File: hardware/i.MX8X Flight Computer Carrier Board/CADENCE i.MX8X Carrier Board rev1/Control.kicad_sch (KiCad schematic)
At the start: 9 parts, among them SW1 SW_DIP_x04, SW2 KMR221GLFS, SW3 SW_DIP_x01

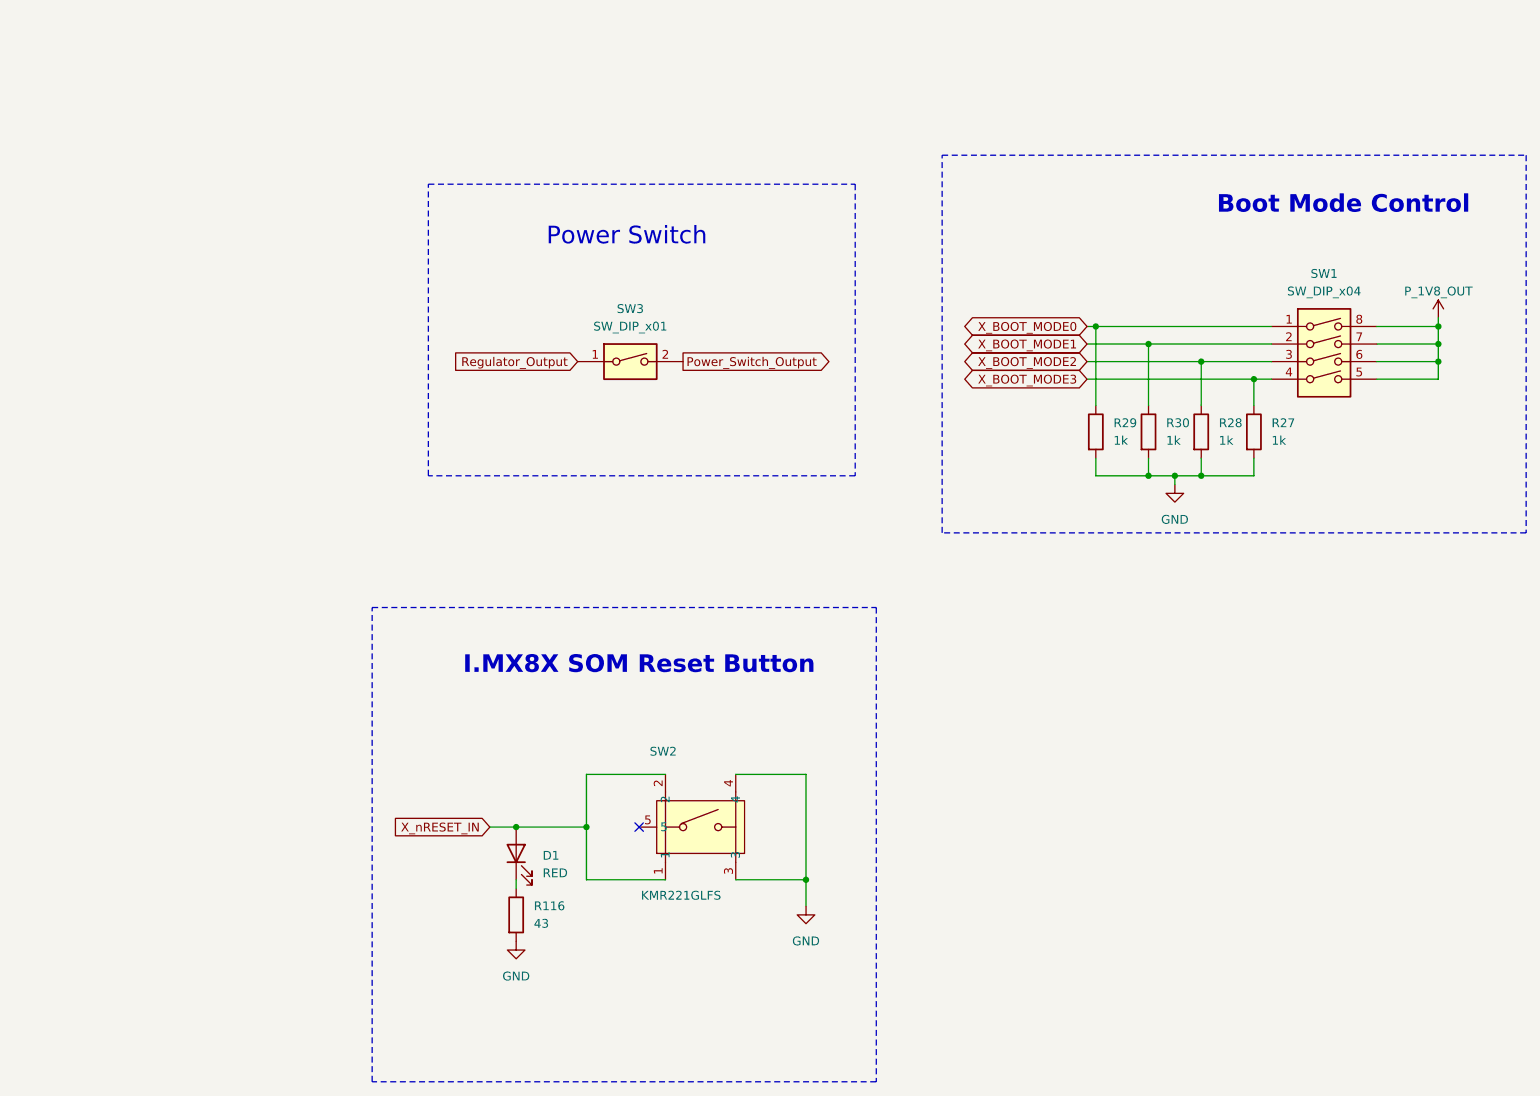
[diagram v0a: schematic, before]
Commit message: schematic reorg
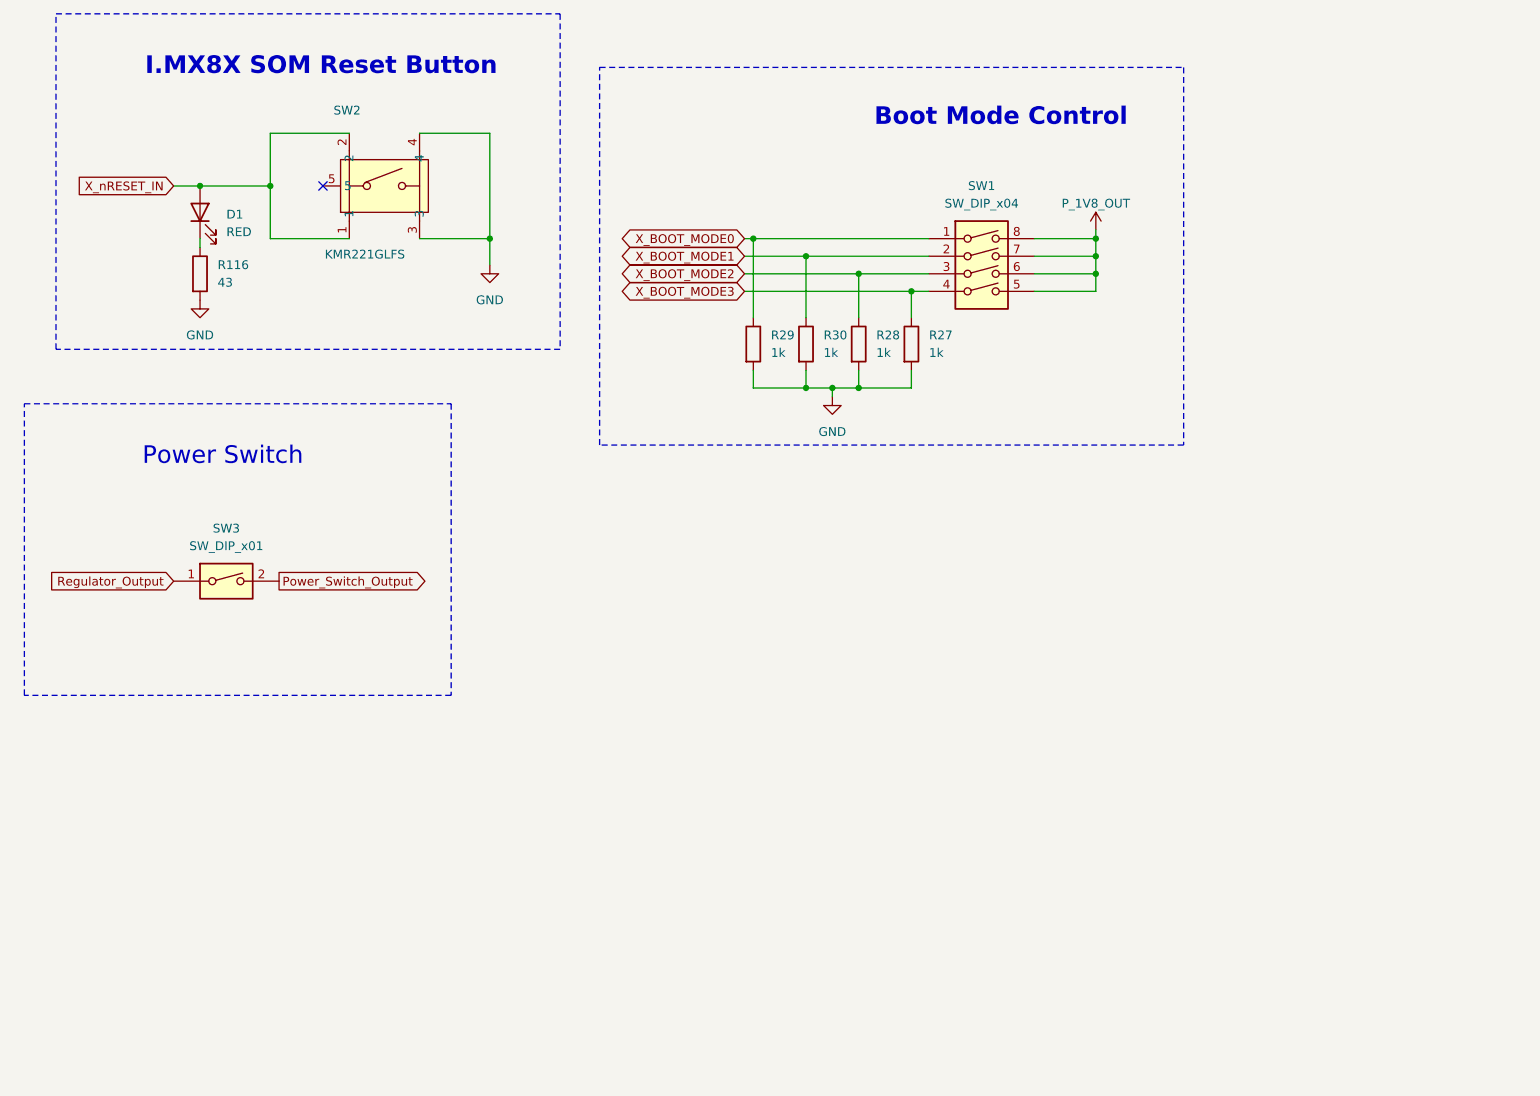
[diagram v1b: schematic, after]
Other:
- moved on the sheet: D1, R116, R27, R28, R29, R30, SW1, SW2, SW3
